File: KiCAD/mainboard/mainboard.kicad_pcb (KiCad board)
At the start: 10 copper layers, 142.5 x 105.5 mm, 240 parts, among them IC1 SN74AUP1G06DCKR, IC3 SN74AUP1G06DCKR, IC4 SN74AUP1G07DCKR, IC5 SN74AUP1G07DCKR, J1 AXT550124, J10 Conn_01x05_Pin, J100 AHDF15A-KG-TAXB, J2 Conn_01x07_Pin, J23 B12B-XH-ALFSN, J29 Conn_01x04_Pin, J3 Conn_02x05_Odd_Even, J30 Conn_01x08_Pin, J31 Conn_01x08_Pin, J4 Conn_01x05_Pin, J5 EJ508B, SW2 100SP1T1B4M2QE, U1 XAL5030-472MEC, U12 ECS-2520MV-xxx-xx, U13 MX25L3233FM2, U14 SN74AUP1G06DCKR, U16 DLPC1438ZEZ, U2 LMR33610BDDAR, U22 TXS0102DCU, U24 DLPA2005ERSLT, U26 TPS54340DDA, U3 LMR33610BDDAR, U37 TXS0102DCU, U38 TPD2E001DRYR, U39 TPS62260DDCT, U4 LMR33610BDDAR, U5 SN74AUP1G06DCKR, U6 74AHC1G08, U7 SN74AUP1G06DCKR, U8 74AHC1G32

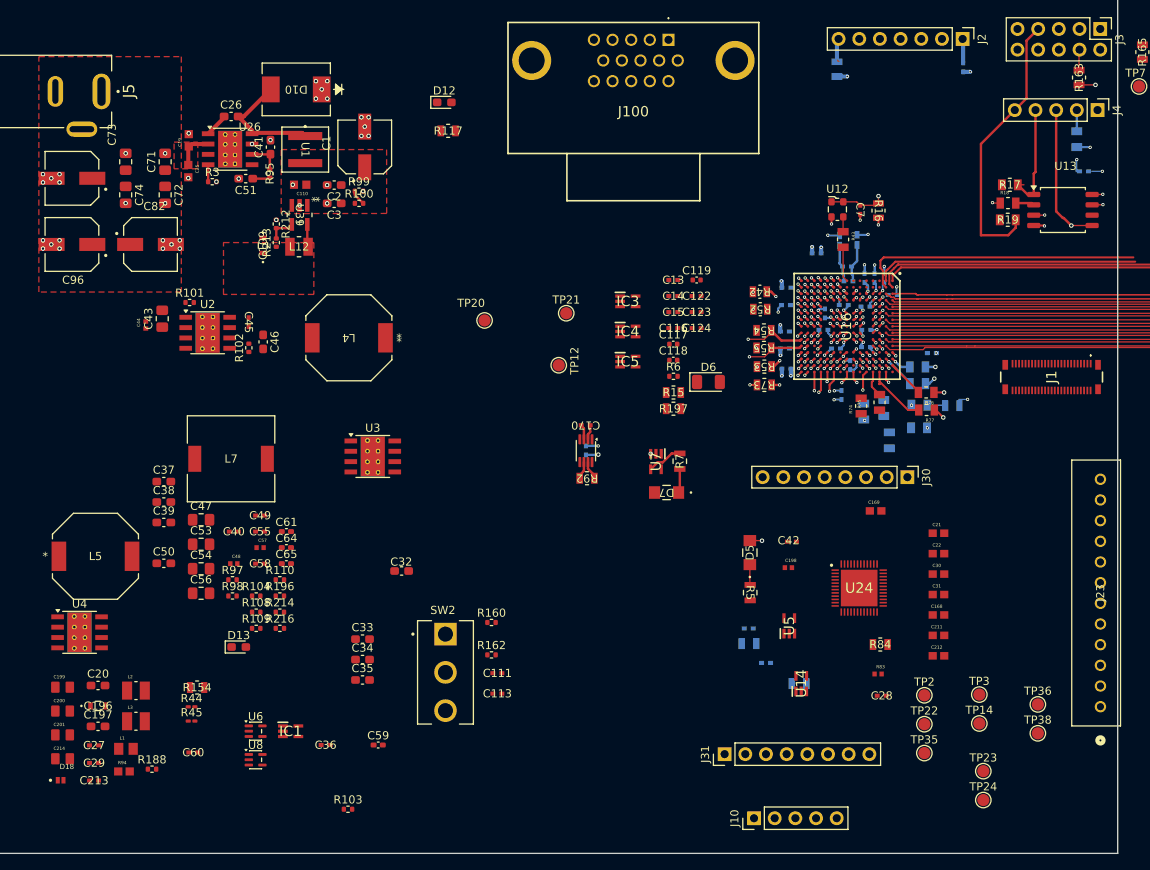
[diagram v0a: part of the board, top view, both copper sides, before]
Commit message: DLPA layout
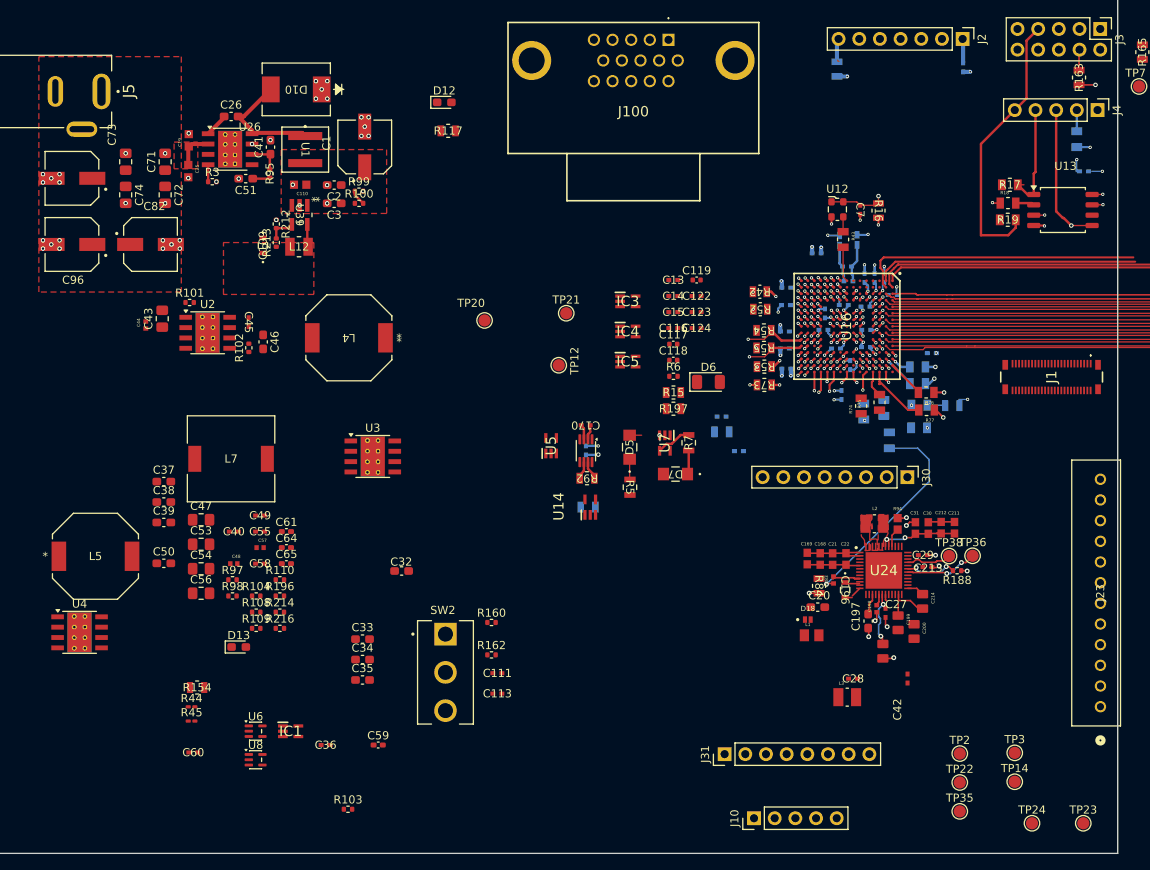
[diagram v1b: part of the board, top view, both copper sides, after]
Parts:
- TP23: value TestPoint -> VOFS
- TP24: value TestPoint -> VBIAS
- TP36: value TestPoint -> SENS2
- TP38: value TestPoint -> SENS1
- moved C214 107.4 mm to (196.2, 120.1), turned to -90 degrees
- moved C213 105.7 mm to (196.8, 115.9)
- moved C200 105.1 mm to (195.1, 123.8), turned to -90 degrees
- moved C29 105.0 mm to (196.2, 114.4)
- moved C199 103.0 mm to (193.2, 122.7), turned to -90 degrees
- moved R188 101.9 mm to (200.4, 116.3), turned to 180 degrees
- moved C201 101.3 mm to (191.3, 126.2), turned to -90 degrees
- moved R94 99.8 mm to (193.1, 110.6), turned to 90 degrees
- moved C27 98.6 mm to (191.6, 121.5), turned to -90 degrees
- moved C197 95.5 mm to (189.5, 122.5), turned to 90 degrees
- moved D18 93.9 mm to (182.1, 122.3)
- moved L2 93.0 mm to (190.2, 110.6), turned to 180 degrees
- moved C196 92.9 mm to (186.7, 118.7), turned to -90 degrees
- moved C20 88.9 mm to (183.3, 120.8)
- moved L3 87.4 mm to (186.9, 131.9)
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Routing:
- net GND: track 67.6 -> 99.5 mm, vias 134 -> 143
- net /DLPC1438_Interface/SPI1_MISO: track 0.50 -> 27.4 mm, vias 1 -> 2
- net P5V: track 0.00 -> 20.1 mm, vias 0 -> 2
- net /DLPA2005_Interface/LED_ANODE: track 0.00 -> 11.4 mm, vias 0 -> 2
- net P3P3V_SB: track 5.97 -> 15.2 mm, vias 6 -> 7
- net /DLPA2005_Interface/SENS2: track 0.00 -> 9.02 mm, vias 0 -> 2
- net Net-(U24-LED_SEL0): track 0.00 -> 6.81 mm, vias 0 -> 2
- net /DLPA2005_Interface/SENS!: track 0.00 -> 5.65 mm
- net /DLPA2005_Interface/PMIC_SPI_DOUT: track 0.00 -> 4.50 mm
- net VBIAS: track 0.00 -> 2.38 mm
- net /DLPA2005_Interface/RLIM: track 0.00 -> 2.35 mm
- net V2V5: track 0.00 -> 1.81 mm
- net VOFS: track 0.00 -> 1.43 mm
- net P3P3V: track 5.34 -> 5.32 mm, vias 2 -> 1
- added copper zone on F.Cu, net (none)
- added copper zone on F.Cu, net /DLPA2005_Interface/L2
- added copper zone on F.Cu, net GND
- added copper zone on In7.Cu, net P3P3V_SB

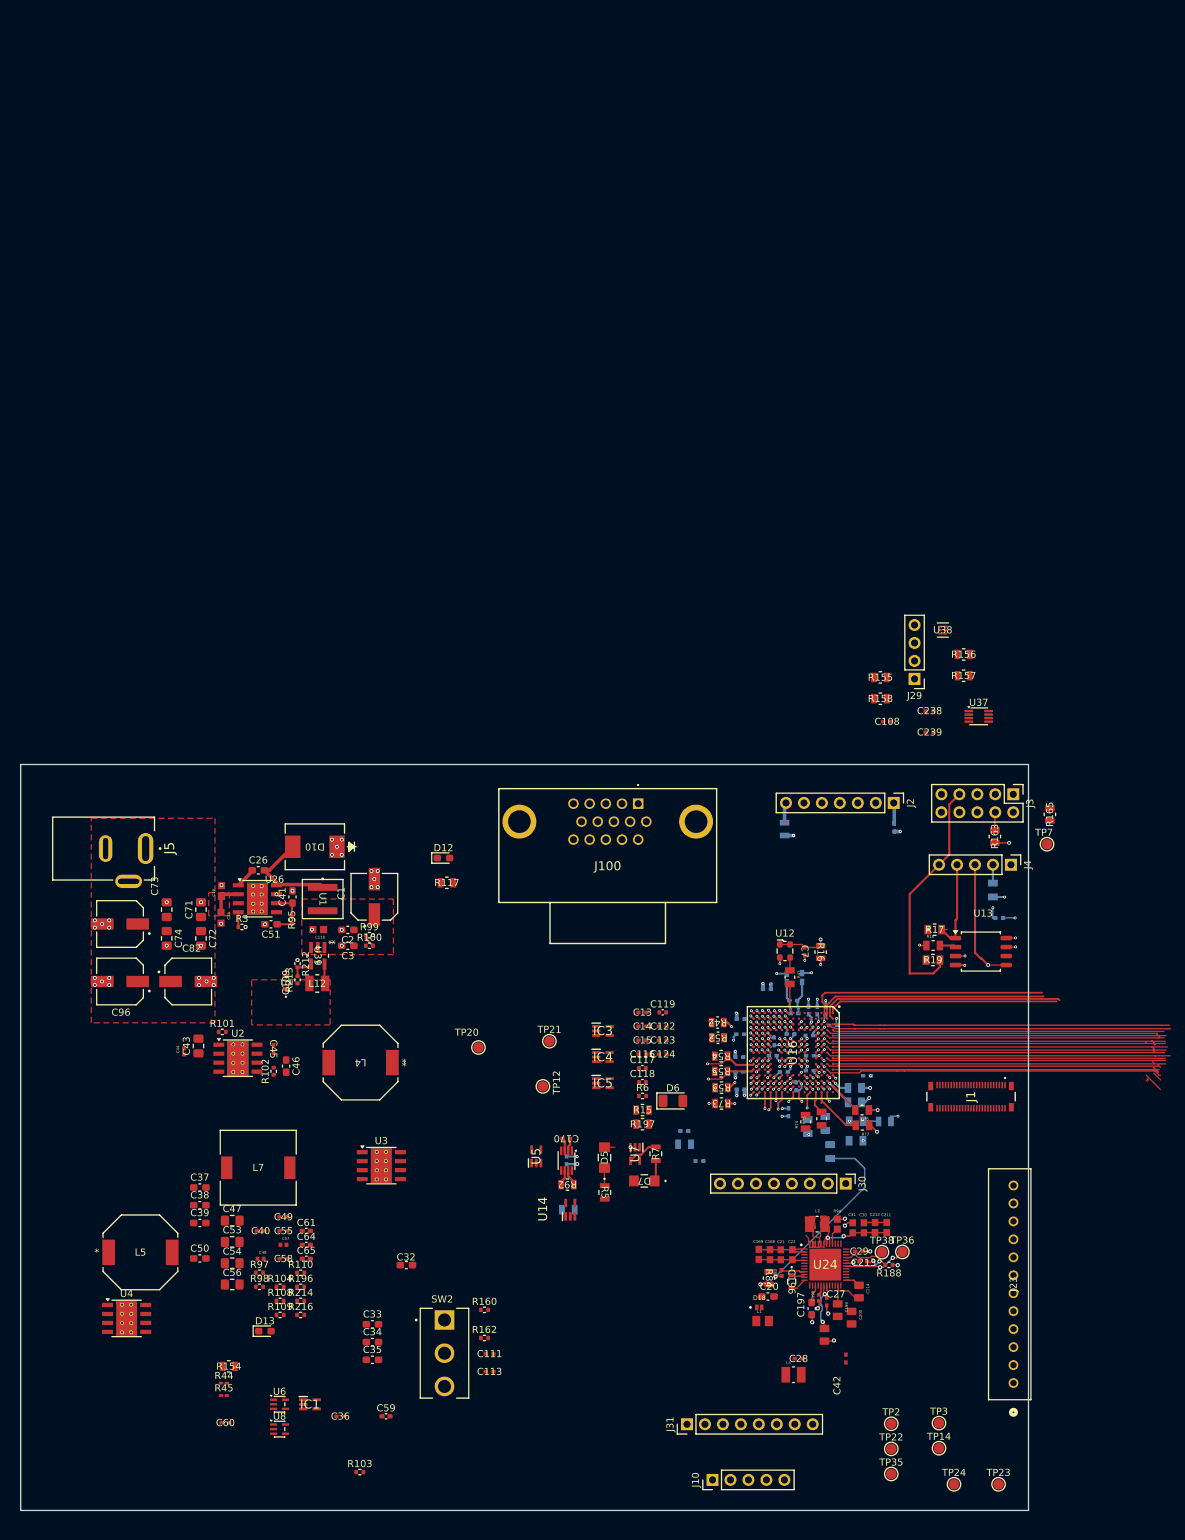
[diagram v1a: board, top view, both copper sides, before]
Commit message: layout
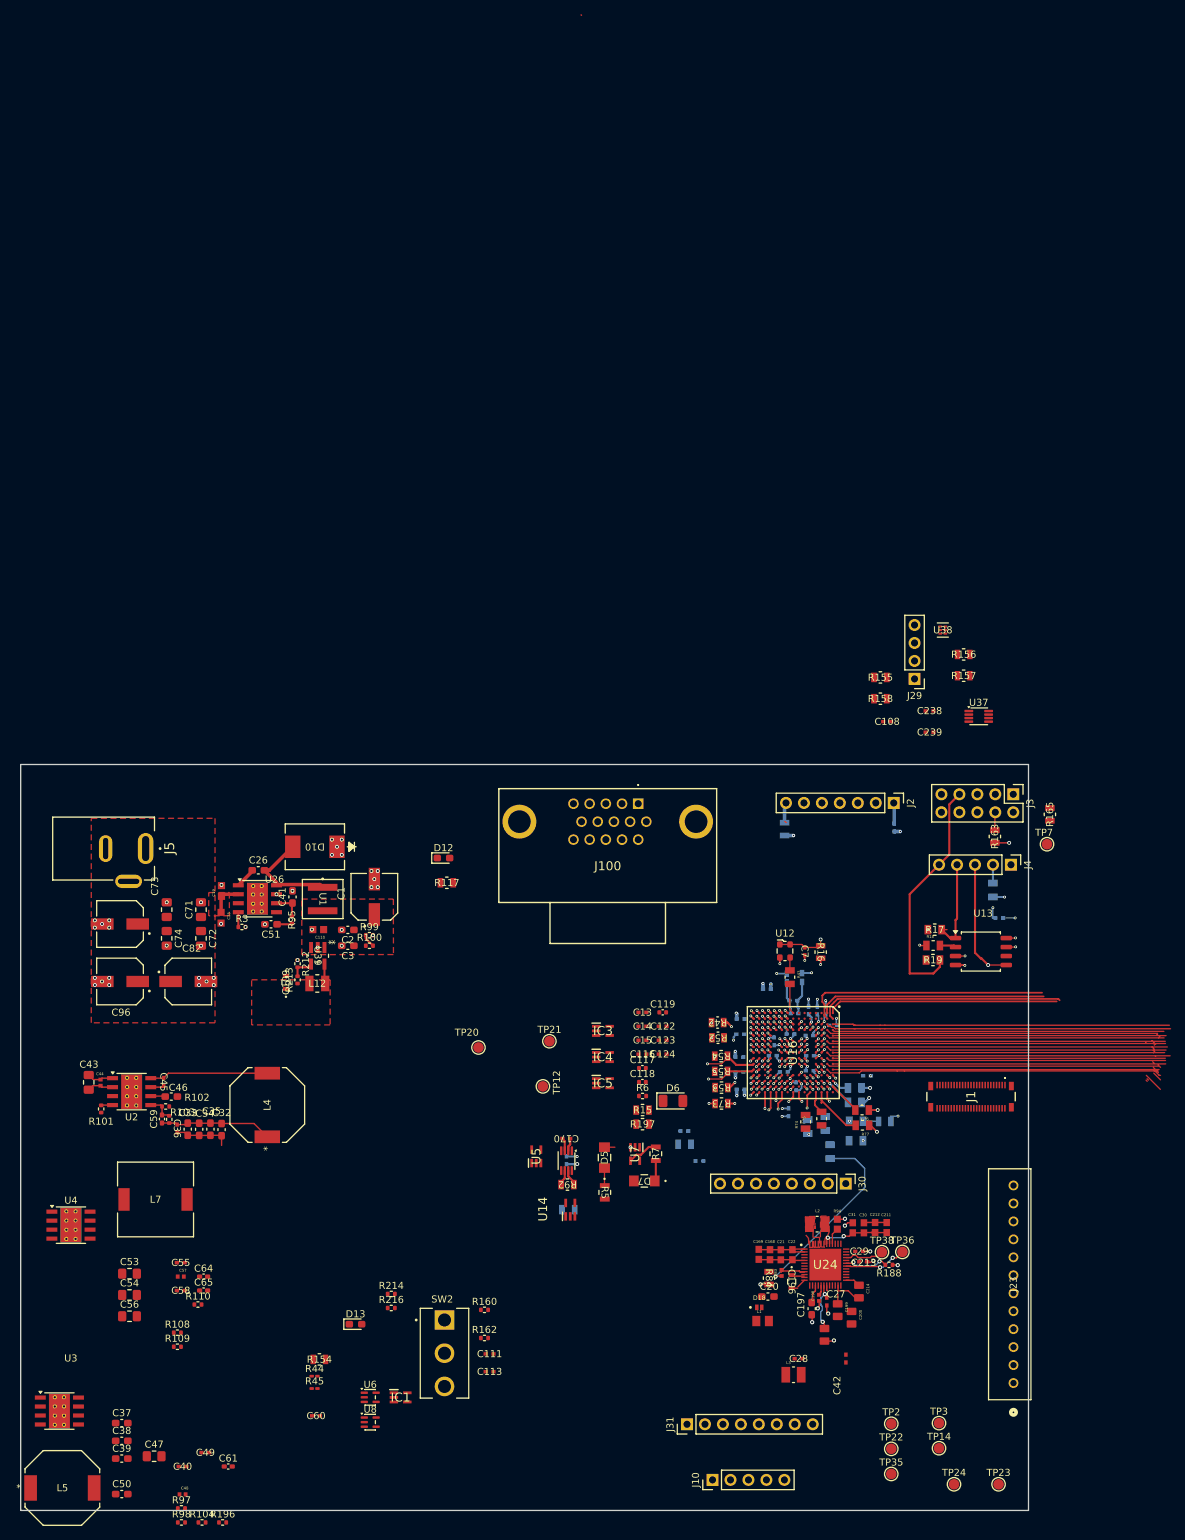
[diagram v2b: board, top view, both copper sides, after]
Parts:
- moved U3 57.2 mm to (83.1, 137.0)
- moved R103 56.7 mm to (98.6, 95.8), turned to 90 degrees
- moved C59 52.7 mm to (97.6, 95.7), turned to 90 degrees
- moved C36 46.8 mm to (99.7, 97.0), turned to -90 degrees
- moved C35 39.9 mm to (104.5, 97.1), turned to -90 degrees
- moved C34 38.8 mm to (102.9, 97.2), turned to -90 degrees
- moved C33 38.0 mm to (101.2, 97.1), turned to -90 degrees
- moved C37 35.1 mm to (91.9, 138.7)
- moved C38 35.1 mm to (91.9, 141.2)
- moved C47 35.1 mm to (96.5, 143.4)
- moved C50 35.1 mm to (91.9, 148.7)
- moved R97 35.1 mm to (100.4, 150.8)
- moved C40 35.1 mm to (100.5, 144.8)
- moved C48 35.1 mm to (100.5, 148.8)
- moved R104 35.1 mm to (103.3, 152.8)
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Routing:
- net /Power_Input&Generation/P1P2V_SW: track 0.00 -> 16.8 mm
- net P1P2V: track 0.00 -> 15.9 mm
- net GND: track 99.5 -> 111.2 mm
- net /Power_Input&Generation/P1P2V_FB: track 0.00 -> 3.97 mm
- net EXT_VIN: track 4.54 -> 8.23 mm
- net /Power_Input&Generation/P1P2V_VCC: track 0.00 -> 2.07 mm
- net /Power_Input&Generation/P1P2V_BOOT: track 0.00 -> 1.91 mm
- net /Power_Input&Generation/P1P2V_PG: track 0.00 -> 1.62 mm

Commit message: layout
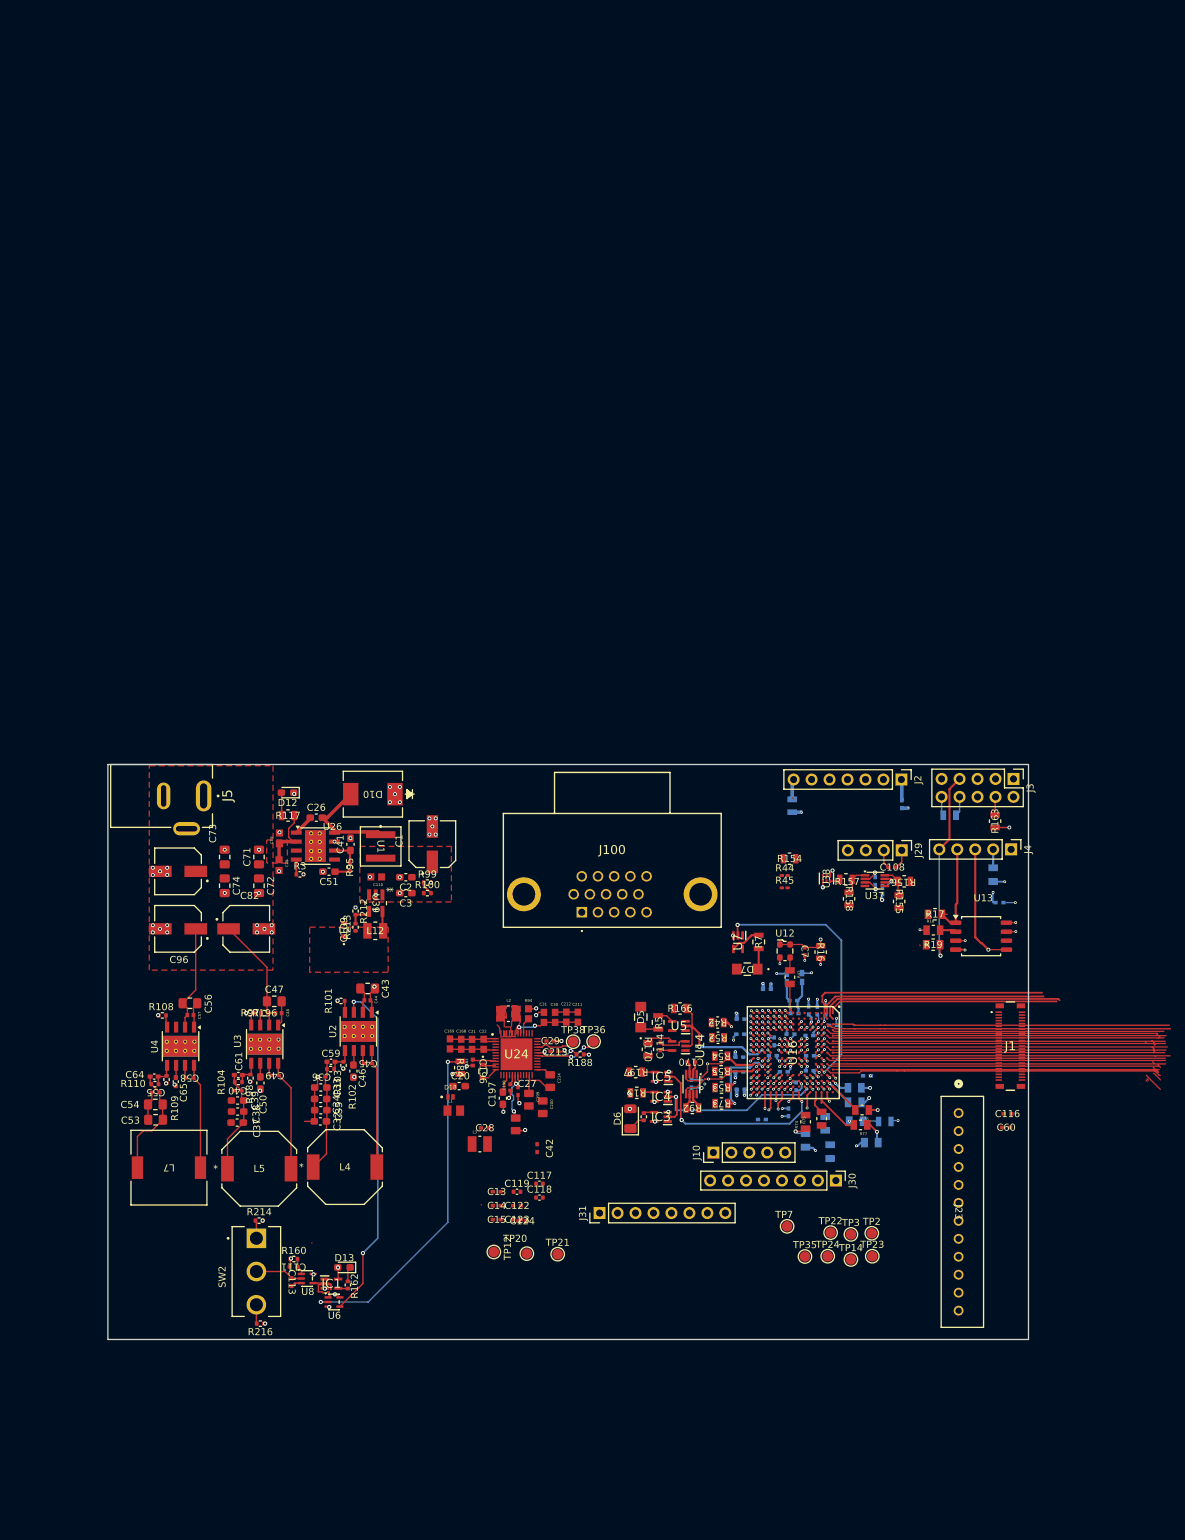
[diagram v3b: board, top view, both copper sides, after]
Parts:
- C114, R166, R170: moved to F.Cu
- C238, C239, R165: moved to B.Cu
- moved C60 105.8 mm to (217.0, 96.9)
- moved R154 97.1 mm to (186.4, 58.9)
- moved R44 97.1 mm to (185.7, 61.3)
- moved R45 97.1 mm to (185.7, 63.0)
- moved R196 72.3 mm to (112.1, 80.7), turned to 180 degrees
- moved R97 70.7 mm to (110.1, 80.7), turned to 180 degrees
- moved C48 69.4 mm to (114.1, 80.7)
- moved C47 66.5 mm to (113.5, 79.1)
- moved TP7 65.4 mm to (186.0, 110.9)
- moved R98 63.6 mm to (110.1, 89.9), turned to -90 degrees
- moved R104 62.5 mm to (108.4, 90.5)
- moved C50 61.4 mm to (111.5, 90.6), turned to -90 degrees
- moved U3 59.5 mm to (112.1, 85.1), turned to -90 degrees
- moved C61 55.4 mm to (108.4, 89.5)
- moved L3 55.1 mm to (142.6, 99.2)
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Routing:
- net /Power_Input&Generation/FPGA_PWREN: track 0.00 -> 48.8 mm, vias 0 -> 2
- net /DLPC1438_Interface/INTZ: track 0.51 -> 48.7 mm, vias 1 -> 3
- net EXT_VIN: track 8.23 -> 45.1 mm
- net /DLPC1438_Interface/RESETZ: track 0.53 -> 37.3 mm, vias 1 -> 2
- net GND: track 111.2 -> 142.6 mm, vias 143 -> 162
- net GPIO_6: track 0.48 -> 27.4 mm, vias 1 -> 2
- net GPIO_9: track 1.47 -> 28.2 mm, vias 1 -> 2
- net /DLPC1438_Interface/SPI1_MISO: track 27.4 -> 1.41 mm
- net /DLPC1438_Interface/DLPC_HOST_IRQ: track 0.58 -> 22.6 mm, vias 1 -> 2
- net P1P8V: track 0.00 -> 17.3 mm, vias 0 -> 1
- net /Power_Input&Generation/P1P8V_SW: track 0.00 -> 15.7 mm
- net /Power_Input&Generation/P3P3V_SW: track 0.00 -> 14.9 mm
- net P3P3V: track 5.32 -> 20.2 mm, vias 1 -> 4
- net /DLPC1438_Interface/IIC0_SCL: track 1.53 -> 11.8 mm
- net /DLPA2005_Interface/PROJ_ON: track 0.00 -> 9.52 mm
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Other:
- board size 142.5 x 105.5 mm -> 130.2 x 81.3 mm
